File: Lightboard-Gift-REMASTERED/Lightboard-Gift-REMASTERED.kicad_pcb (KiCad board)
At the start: 2 copper layers, 90 x 62 mm, 20 parts, among them J1 USB_C_Receptacle_PowerOnly_6P, SW1 SW_Push, SW2 SW_SPST

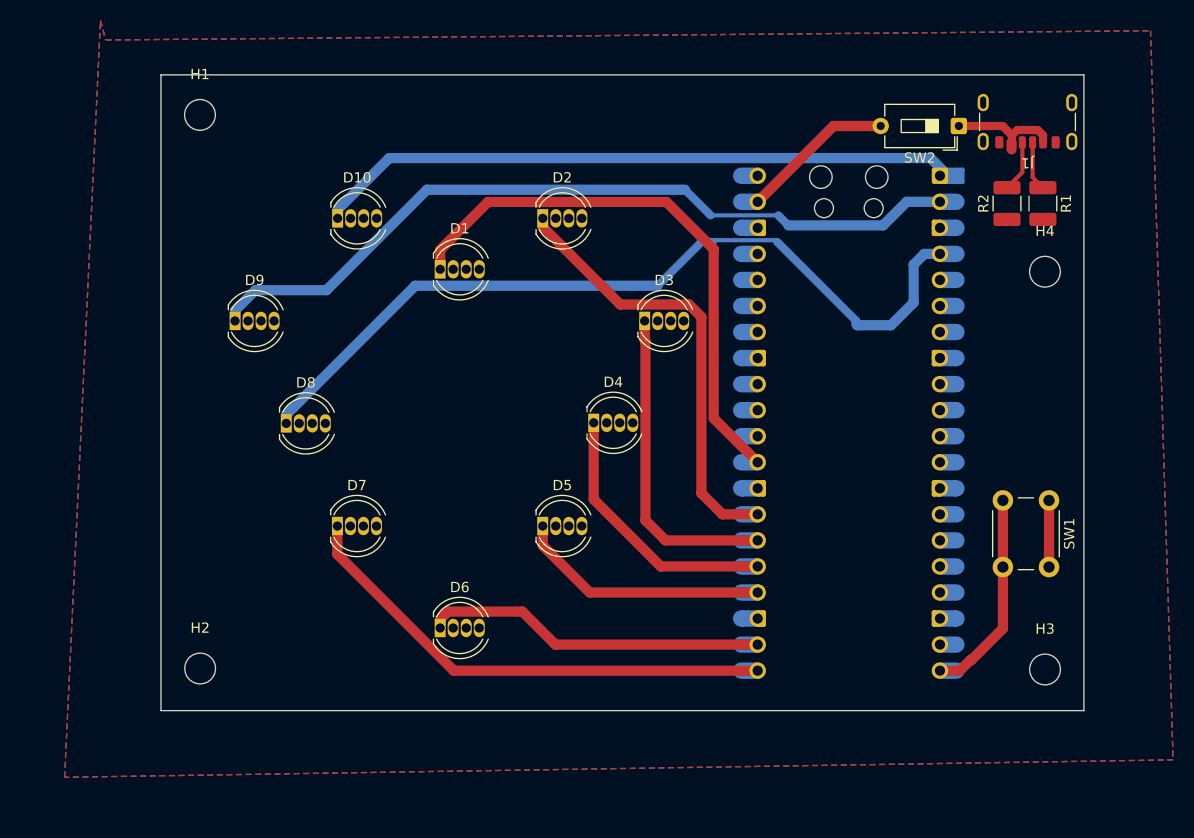
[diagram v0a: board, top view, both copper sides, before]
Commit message: Work Hard Play Harder
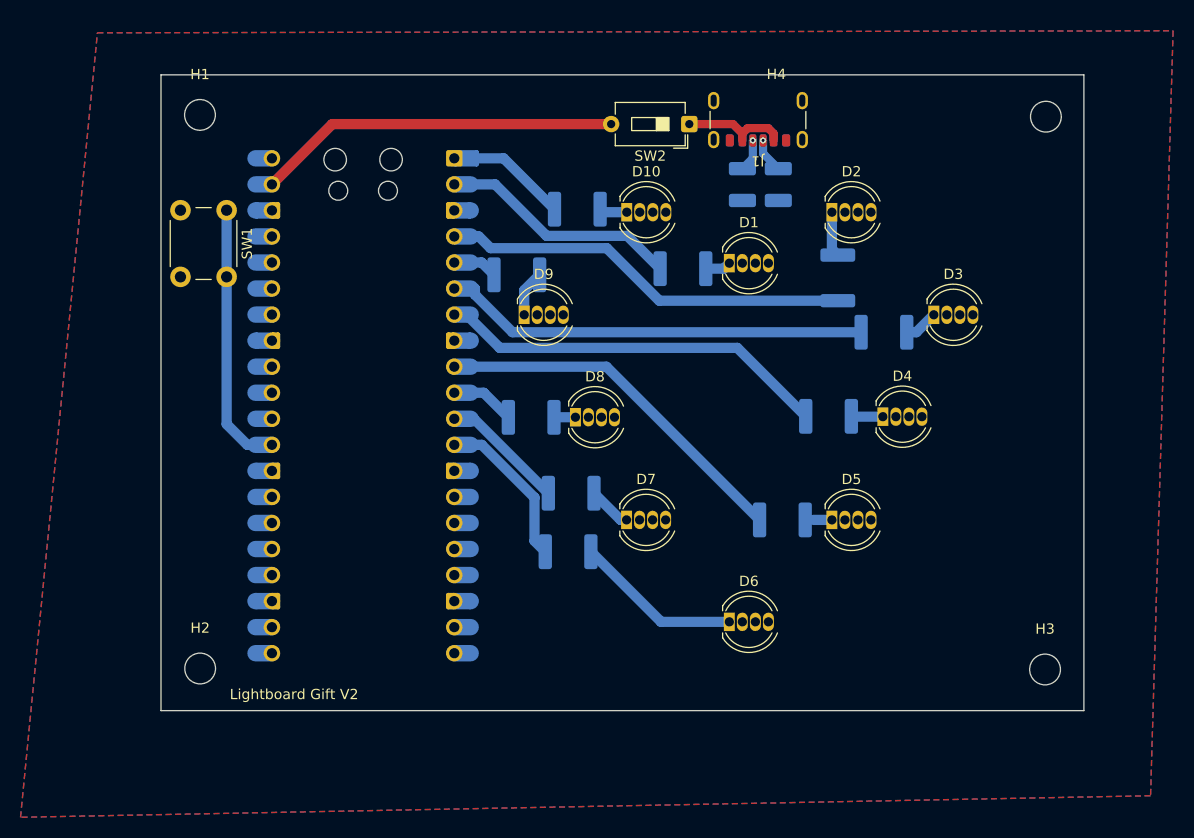
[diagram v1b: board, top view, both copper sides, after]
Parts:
- added R10: R_Small, Resistor_SMD:R_1812_4532Metric_Pad1.30x3.40mm_HandSolder, B.Cu at (137.6, 89.4)
- added R11: R_Small, Resistor_SMD:R_1812_4532Metric_Pad1.30x3.40mm_HandSolder, B.Cu at (136.2, 75.5)
- added R12: R_Small, Resistor_SMD:R_1812_4532Metric_Pad1.30x3.40mm_HandSolder, B.Cu at (142.1, 69.1)
- added R3: R_Small, Resistor_SMD:R_1812_4532Metric_Pad1.30x3.40mm_HandSolder, B.Cu at (152.4, 74.9)
- added R4: R_Small, Resistor_SMD:R_1812_4532Metric_Pad1.30x3.40mm_HandSolder, B.Cu at (167.5, 75.8)
- added R5: R_Small, Resistor_SMD:R_1812_4532Metric_Pad1.30x3.40mm_HandSolder, B.Cu at (172.0, 81.1)
- added R6: R_Small, Resistor_SMD:R_1812_4532Metric_Pad1.30x3.40mm_HandSolder, B.Cu at (166.6, 89.3)
- added R7: R_Small, Resistor_SMD:R_1812_4532Metric_Pad1.30x3.40mm_HandSolder, B.Cu at (162.1, 99.4)
- added R8: R_Small, Resistor_SMD:R_1812_4532Metric_Pad1.30x3.40mm_HandSolder, B.Cu at (141.2, 102.5)
- added R9: R_Small, Resistor_SMD:R_1812_4532Metric_Pad1.30x3.40mm_HandSolder, B.Cu at (141.5, 96.8)
- R1, R2: moved to B.Cu
- moved SW1 85.0 mm to (107.9, 69.2)
- moved A1 47.4 mm to (121.2, 88.3)
- moved D8 28.2 mm to (141.9, 89.4)
- moved D1 28.2 mm to (156.9, 74.4)
- moved D2 28.2 mm to (166.9, 69.4)
- moved D3 28.2 mm to (176.9, 79.4)
- moved D5 28.2 mm to (166.9, 99.4)
- moved D6 28.2 mm to (156.9, 109.3)
- moved D7 28.2 mm to (146.9, 99.4)
- moved D9 28.2 mm to (136.9, 79.4)
- moved D10 28.2 mm to (146.9, 69.4)
- moved D4 28.2 mm to (171.9, 89.3)
- moved J1 26.3 mm to (159.7, 59.3)
- moved SW2 26.3 mm to (153.0, 60.8)
- moved R1 25.9 mm to (161.7, 66.7)
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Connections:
- A1 pad 10: unconnected-(A1-GPIO7-Pad10) -> RED7
- A1 pad 11: unconnected-(A1-GPIO8-Pad11) -> RED6
- A1 pad 12: unconnected-(A1-GPIO9-Pad12) -> RED5
- A1 pad 13: Net-(A1-GND-Pad13) -> GND
- A1 pad 18: Net-(A1-GND-Pad13) -> GND
- A1 pad 2: RED8 -> RED0
- A1 pad 20: Net-(A1-GPIO15) -> unconnected-(A1-GPIO15-Pad20)
- A1 pad 21: RED6 -> unconnected-(A1-GPIO16-Pad21)
- A1 pad 22: RED5 -> unconnected-(A1-GPIO17-Pad22)
- A1 pad 23: Net-(A1-GND-Pad13) -> GND
- A1 pad 24: RED4 -> unconnected-(A1-GPIO18-Pad24)
- A1 pad 25: RED3 -> unconnected-(A1-GPIO19-Pad25)
- A1 pad 26: RED2 -> unconnected-(A1-GPIO20-Pad26)
- A1 pad 27: RED1 -> unconnected-(A1-GPIO21-Pad27)
- A1 pad 28: Net-(A1-GND-Pad13) -> GND
- A1 pad 29: RED0 -> Net-(A1-GPIO22)
- A1 pad 3: Net-(A1-GND-Pad13) -> GND
- A1 pad 33: unconnected-(A1-AGND-Pad33) -> GND
- A1 pad 38: Net-(A1-GND-Pad13) -> GND
- A1 pad 4: RED7 -> RED1
- A1 pad 5: unconnected-(A1-GPIO3-Pad5) -> RED8
- A1 pad 6: unconnected-(A1-GPIO4-Pad6) -> RED2
- A1 pad 7: unconnected-(A1-GPIO5-Pad7) -> RED3
- A1 pad 8: Net-(A1-GND-Pad13) -> GND
- A1 pad 9: unconnected-(A1-GPIO6-Pad9) -> RED4
- D1 pad 1: RED0 -> Net-(D1-RA)
- D10 pad 1: RED9 -> Net-(D10-RA)
- D2 pad 1: RED1 -> Net-(D2-RA)
- D3 pad 1: RED2 -> Net-(D3-RA)
- D4 pad 1: RED3 -> Net-(D4-RA)
- D5 pad 1: RED4 -> Net-(D5-RA)
- D6 pad 1: RED5 -> Net-(D6-RA)
- D7 pad 1: RED6 -> Net-(D7-RA)
- D8 pad 1: RED7 -> Net-(D8-RA)
- D9 pad 1: RED8 -> Net-(D9-RA)
- SW1 pad 1: GND -> Net-(A1-GPIO22)
- SW1 pad 2: Net-(A1-GPIO15) -> GND
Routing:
- net RED7: track 81.1 -> 5.47 mm
- net RED8: track 77.0 -> 3.57 mm
- net RED9: track 63.2 -> 11.0 mm
- net RED6: track 48.4 -> 11.4 mm
- net RED0: track 55.0 -> 22.7 mm
- net Net-(A1-GPIO22): track 0.00 -> 25.3 mm
- net VBUS: track 15.1 -> 35.5 mm
- net Net-(A1-GPIO15): track 20.3 -> 0.00 mm
- net RED5: track 33.4 -> 14.9 mm
- net Net-(D6-RA): track 0.00 -> 16.3 mm
- net RED3: track 26.2 -> 37.6 mm
- net RED4: track 24.8 -> 35.2 mm
- net RED2: track 31.2 -> 41.0 mm
- net GND: track 6.50 -> 0.00 mm
- net Net-(D9-RA): track 0.00 -> 4.52 mm
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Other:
- board text added: "Lightboard Gift V2"
